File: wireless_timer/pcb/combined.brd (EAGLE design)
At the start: 36 x 76.5 mm, 66 parts, among them U1 1, U2 TPS, U3 PMOS, U4 PMOS

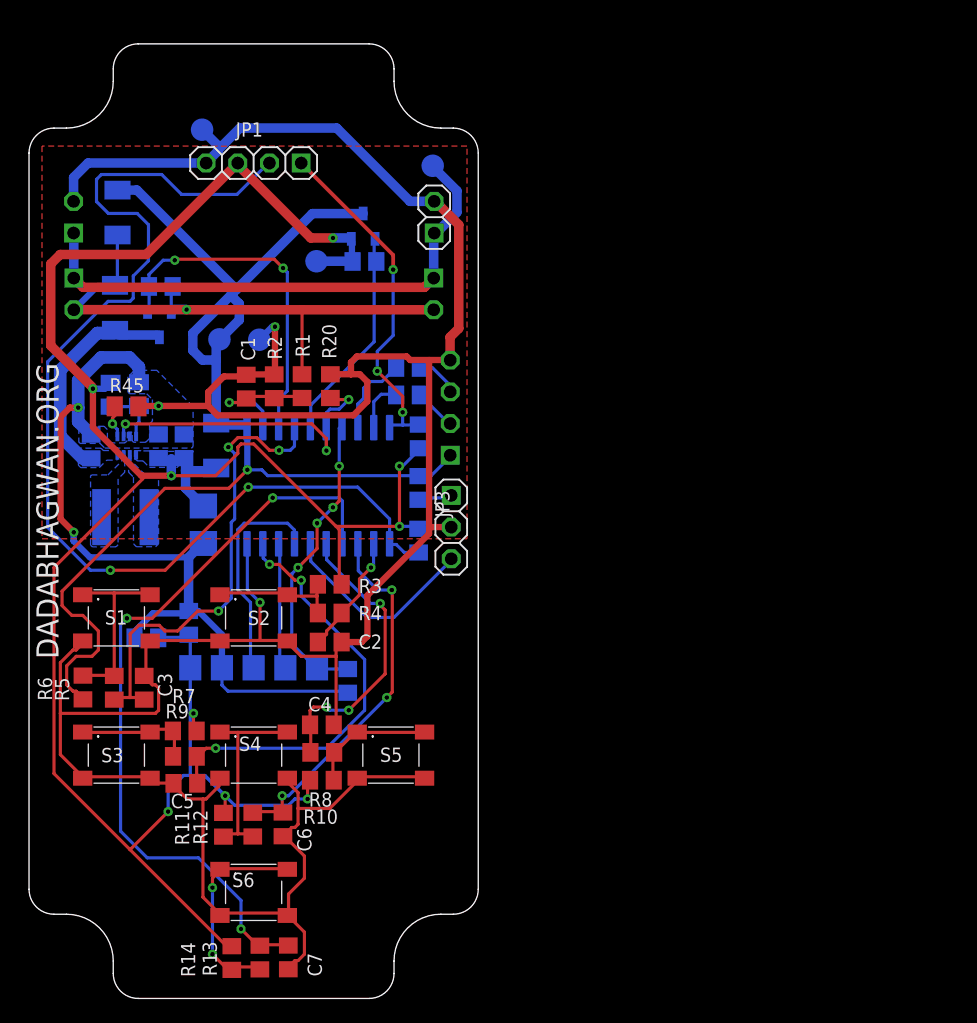
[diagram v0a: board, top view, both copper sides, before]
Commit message: panel made, outline pending
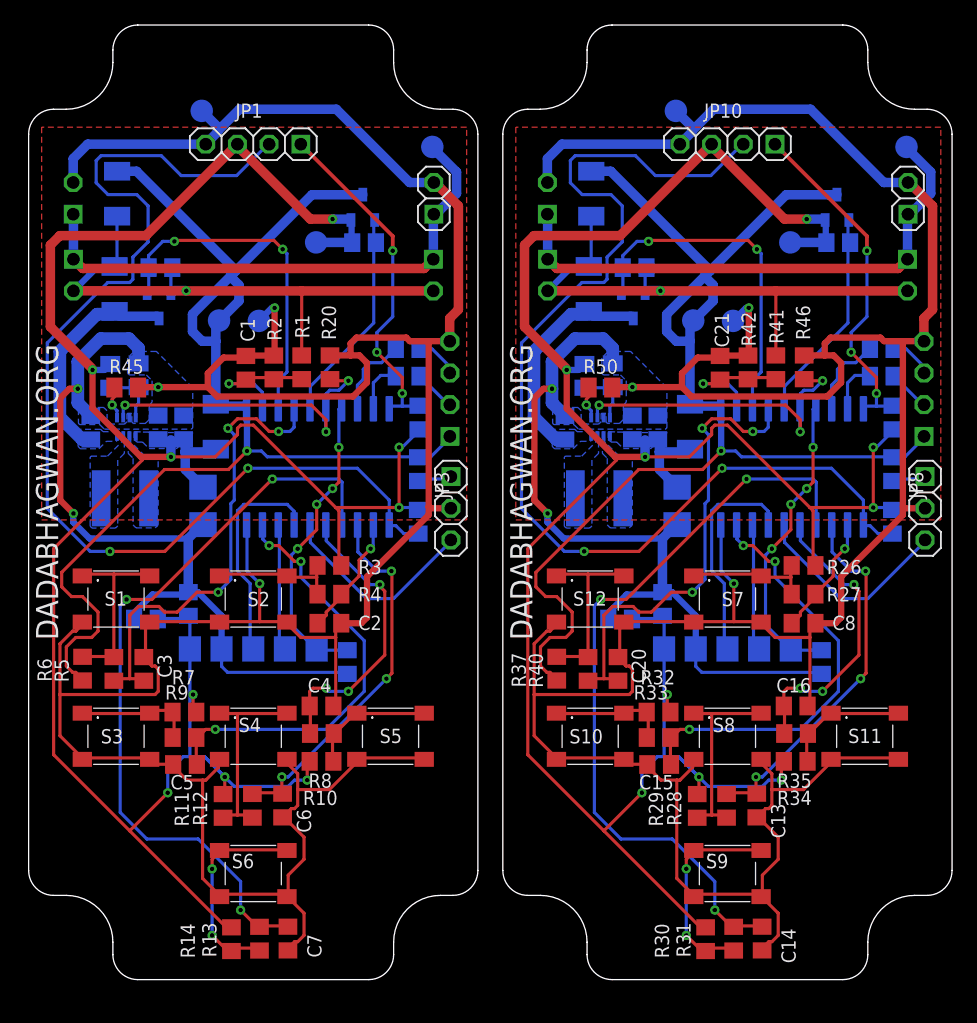
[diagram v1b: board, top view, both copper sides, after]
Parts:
- added A2: 1X05, pinhead_smd:1X05X254
- added C12: 10uF, rcl:CT3528
- added C13, C14, C15, C16, C20, C21, C8: 100nF, rcl:C0805
- added C22, C23, C24, C25, C26: 10uF, rcl:C0805
- added D4, D5, D6: BAT, diode:SOD-123_MINI-SMA
- added JP10, JP9: (no value), pinhead-2:1X04-S
- added JP11, JP12, JP13, JP14: (no value), pinhead-2:1X02-S
- added JP8: (no value), pinhead-2:1X03-S
- added L2: 1uH, 5040_INDUCTOR:IND_74404043220A
- added R24, R25, R36, R46: 30K, rcl:R0805
- added R26, R27, R28, R29, R30, R31, R32, R33, R34, R35, R37, R40: 10K, rcl:R0805
- added R41, R42, R51, R52: 100K, rcl:R0805
- added R43, R44: 1K, rcl:R0805
- added R47: 200E, rcl:R0805
- added R48: 511K, rcl:M0805
- added R49: 91K, rcl:M0805
- added R50: 50K, rcl:M0805
- added S10, S11, S12, S7, S8, S9: SW, switch_5p5mm:SW_55MM
- added TP10: VCC, testpad:TP18R
- added TP6: VBAT, testpad:TP18R
- added TP7, TP8: GND, testpad:TP18R
- added TP9: VDD, testpad:TP18R
- added U5: 1, ATTINY1616-SNR:SOIC127P1032X265-20N
- added U6: TPS, TPS63000DRLR:SOTFL50P160X60-8N
- added U7, U8: PMOS, DMP3165L:SOT103P240X110-3N
- moved C9 1.51 mm to (14.0, 38.0)
- moved D2 1.51 mm to (15.0, 44.3)
- moved JP1 1.51 mm to (18.0, 67.0)
- moved JP5 1.51 mm to (33.8, 47.3)
- moved R2 1.51 mm to (19.6, 49.1)
- moved R22 1.51 mm to (10.6, 57.1)
- moved R23 1.51 mm to (26.9, 59.1)
- moved R38 1.51 mm to (6.54, 48.4)
- moved R45 1.51 mm to (7.82, 47.5)
- moved TP1 1.51 mm to (13.9, 69.6)
- moved TP4 1.51 mm to (32.4, 66.7)
- moved A1 1.51 mm to (18.0, 26.5)
- moved C10 1.51 mm to (12.8, 30.1)
- moved R4 1.51 mm to (24.1, 30.9)
- moved R6 1.51 mm to (4.32, 24.9)
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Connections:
- new net DC_SW1: R51.1, U5.3, U7.1
- new net GND1: A2.2, C12.-, C13.2, C14.2, C15.2, C16.2, C20.2, C21.2, C22.2, C23.2, C24.2, C25.2, C26.2, C8.2, JP10.4, JP11.2, JP12.2, JP8.2, JP9.4, R36.1, R42.2, R46.1, R49.1, R50.1, S10.3, S10.4, S11.3, S11.4, S12.3, S12.4, S7.3, S7.4, S8.3, S8.4, S9.3, S9.4, TP7.TP, TP8.TP, U5.20, U6.7
- new net LX3: L2.2, U6.3
- new net LX4: L2.1, U6.2
- new net N$11: R32.1, R33.2, S10.1, S10.2
- new net N$13: R34.1, R35.2, S11.1, S11.2
- new net N$14: R37.1, R40.2, S12.1, S12.2
- new net N$15: JP8.3, U5.16
- new net N$16: JP8.1, R47.2
- new net N$17: R48.1, R49.2, U6.8
- new net N$18: R50.2, U6.5
- new net N$4: R26.1, R27.2, S7.1, S7.2
- new net N$6: R28.1, R29.2, S8.1, S8.2
- new net N$7: R30.1, R31.2, S9.1, S9.2
- new net RXD02: R44.2, U5.8
- new net RXD03: A2.4, U5.18
- new net RXD04: JP9.3, R44.1
- new net S10: C15.1, R33.1, U5.19
- new net S11: C16.1, R35.1, U5.15
- new net S12: C20.1, R40.1, U5.4
- new net S7: C8.1, R27.1, U5.12
- new net S8: C13.1, R29.1, U5.13
- new net S9: C14.1, R31.1, U5.14
- new net SCL1: JP10.2, R25.2, U5.11
- new net SDA1: JP10.1, R24.2, U5.10
- new net SET1: A2.5, R36.2, U5.7
- new net SHDN1: R46.2, U5.6, U6.6
- new net TXD02: R43.2, U5.9
- new net TXD03: A2.3, U5.17
- new net TXD04: JP9.2, R43.1
- new net VADC1: C21.1, R41.1, R42.1, U5.2
- new net VBAT1: JP11.1, JP12.1, JP13.1, JP14.1, TP6.TP
- new net VBAT_O1: D4.A, D6.A, JP13.2, JP14.2, R41.2, R51.2, U7.2
- new net VCC1: A2.1, C12.+, C22.1, C23.1, C25.1, C26.1, D5.A, JP10.3, R24.1, R25.1, R26.2, R28.2, R30.2, R32.2, R34.2, R48.2, R52.1, TP10.TP, U6.1, U8.2
- new net VCC_SW1: R52.2, U5.5, U8.1
- new net VDD1: D4.C, D5.C, JP9.1, R37.2, R47.1, TP9.TP, U5.1, U8.3
- new net VIN1: C24.1, D6.C, U6.4, U7.3
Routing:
- net GND1: track 0.00 -> 307.2 mm, vias 0 -> 5
- net VCC1: track 0.00 -> 191.0 mm, vias 0 -> 9
- net VDD1: track 0.00 -> 100.5 mm, vias 0 -> 1
- net SCL1: track 0.00 -> 88.3 mm, vias 0 -> 2
- net S9: track 0.00 -> 60.7 mm, vias 0 -> 3
- net VBAT_O1: track 0.00 -> 45.7 mm, vias 0 -> 1
- net VBAT1: track 0.00 -> 43.7 mm
- net S12: track 0.00 -> 37.4 mm, vias 0 -> 3
- net S10: track 0.00 -> 34.6 mm, vias 0 -> 3
- net S8: track 0.00 -> 29.7 mm, vias 0 -> 3
- net SDA1: track 0.00 -> 28.0 mm, vias 0 -> 3
- net DC_SW1: track 0.00 -> 27.8 mm, vias 0 -> 2
- net SHDN1: track 0.00 -> 25.4 mm, vias 0 -> 3
- net SET1: track 0.00 -> 24.4 mm, vias 0 -> 4
- net S11: track 0.00 -> 23.6 mm, vias 0 -> 3
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- added copper zone on layer 1, net GND1
- added copper zone on layer 16, net GND1
- added copper zone on layer 16, net LX3
- added copper zone on layer 16, net LX4
- added copper zone on layer 16, net VCC1
- added copper zone on layer 16, net VIN1
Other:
- board size 36 x 76.5 mm -> 74 x 76.5 mm
- board text added: "A1"
- board text added: "C1"
- board text added: "C10"
- board text added: "C11"
- board text added: "C17"
- board text added: "C18"
- board text added: "C19"
- board text added: "C2"
- board text added: "C3"
- board text added: "C4"
- board text added: "C5"
- board text added: "C6"
- board text added: "C7"
- board text added: "C9"
- board text added: "D1"
- board text added: "D2"
- board text added: "D3"
- board text added: "JP1"
- board text added: "JP2"
- board text added: "JP3"
- board text added: "JP4"
- board text added: "JP5"
- board text added: "JP6"
- board text added: "JP7"
- board text added: "L1"
- board text added: "R1"
- board text added: "R10"
- board text added: "R11"
- board text added: "R12"
- board text added: "R13"
- board text added: "R14"
- board text added: "R15"
- board text added: "R16"
- board text added: "R17"
- board text added: "R18"
- board text added: "R19"
- board text added: "R2"
- board text added: "R20"
- board text added: "R21"
- board text added: "R22"
- board text added: "R23"
- board text added: "R3"
- board text added: "R38"
- board text added: "R39"
- board text added: "R4"
- board text added: "R45"
- board text added: "R5"
- board text added: "R6"
- board text added: "R7"
- board text added: "R8"
- board text added: "R9"
- board text added: "S1"
- board text added: "S2"
- board text added: "S3"
- board text added: "S4"
- board text added: "S5"
- board text added: "S6"
- board text added: "TP1"
- board text added: "TP2"
- board text added: "TP3"
- board text added: "TP4"
- board text added: "TP5"
- board text added: "U1"
- board text added: "U2"
- board text added: "U3"
- board text added: "U4"
